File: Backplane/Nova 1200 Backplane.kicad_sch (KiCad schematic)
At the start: 46 parts, among them J1 Conn_02x40_Odd_Even, J10 Conn_01x10, J11 Conn_01x10, J12 Conn_01x10, J13 Conn_01x10, J14 Conn_01x10, J15 Conn_01x10, J16 Conn_01x10, J17 Conn_01x10, J18 Conn_01x10, J19 Conn_01x10, J1A1 Conn_01x40, J1A2 Conn_01x40, J1A3 Conn_01x40, J1A4 Conn_01x40, J1A5 Conn_01x40, J1B1 Conn_01x40, J1B2 Conn_01x40, J1B3 Conn_01x40, J1B4 Conn_01x40, J1B5 Conn_01x40, J2 DG Nova Card-Edge 81-100, J20 Conn_01x10, J21 Conn_01x10, J22 Conn_01x10, J23 Conn_01x10, J24 Conn_01x10, J2A1 Conn_01x40, J2A2 Conn_01x40, J2A3 Conn_01x40, J2A4 Conn_01x40, J2A5 Conn_01x40, J2B1 Conn_01x40, J2B2 Conn_01x40, J2B3 Conn_01x40, J2B4 Conn_01x40, J2B5 Conn_01x40, J3 Conn_02x40_Odd_Even, J4 DG Nova Card-Edge 81-100, J5 Conn_01x10, J6 Conn_01x10, J7 Conn_01x10, J8 Conn_01x10, J9 Conn_01x10

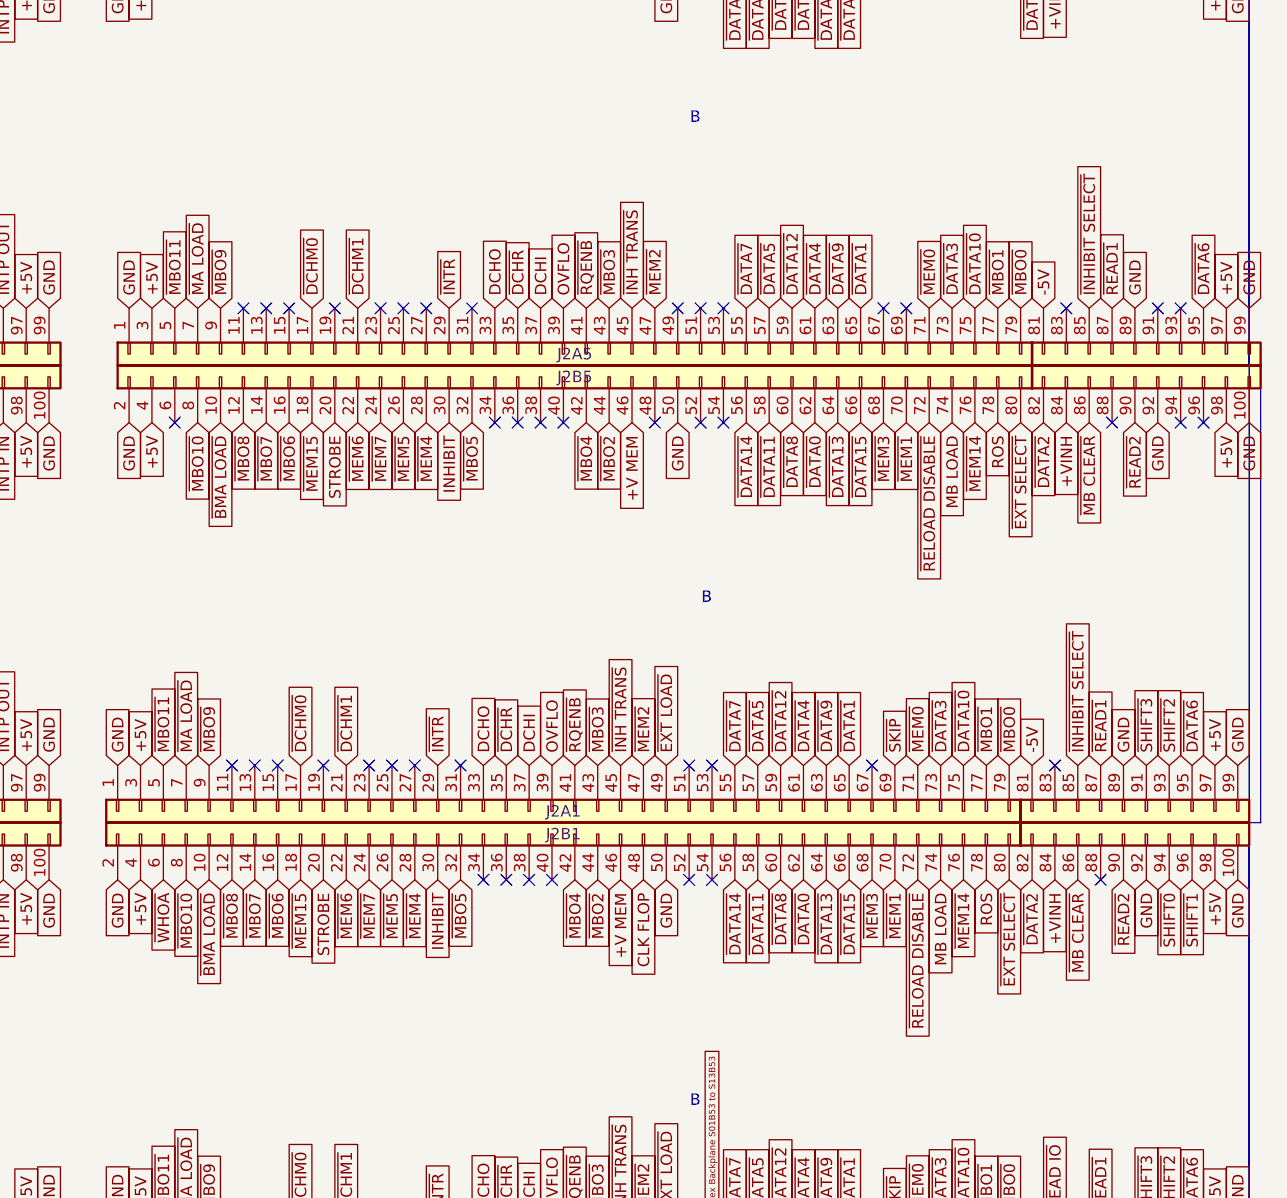
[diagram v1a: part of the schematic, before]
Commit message: more
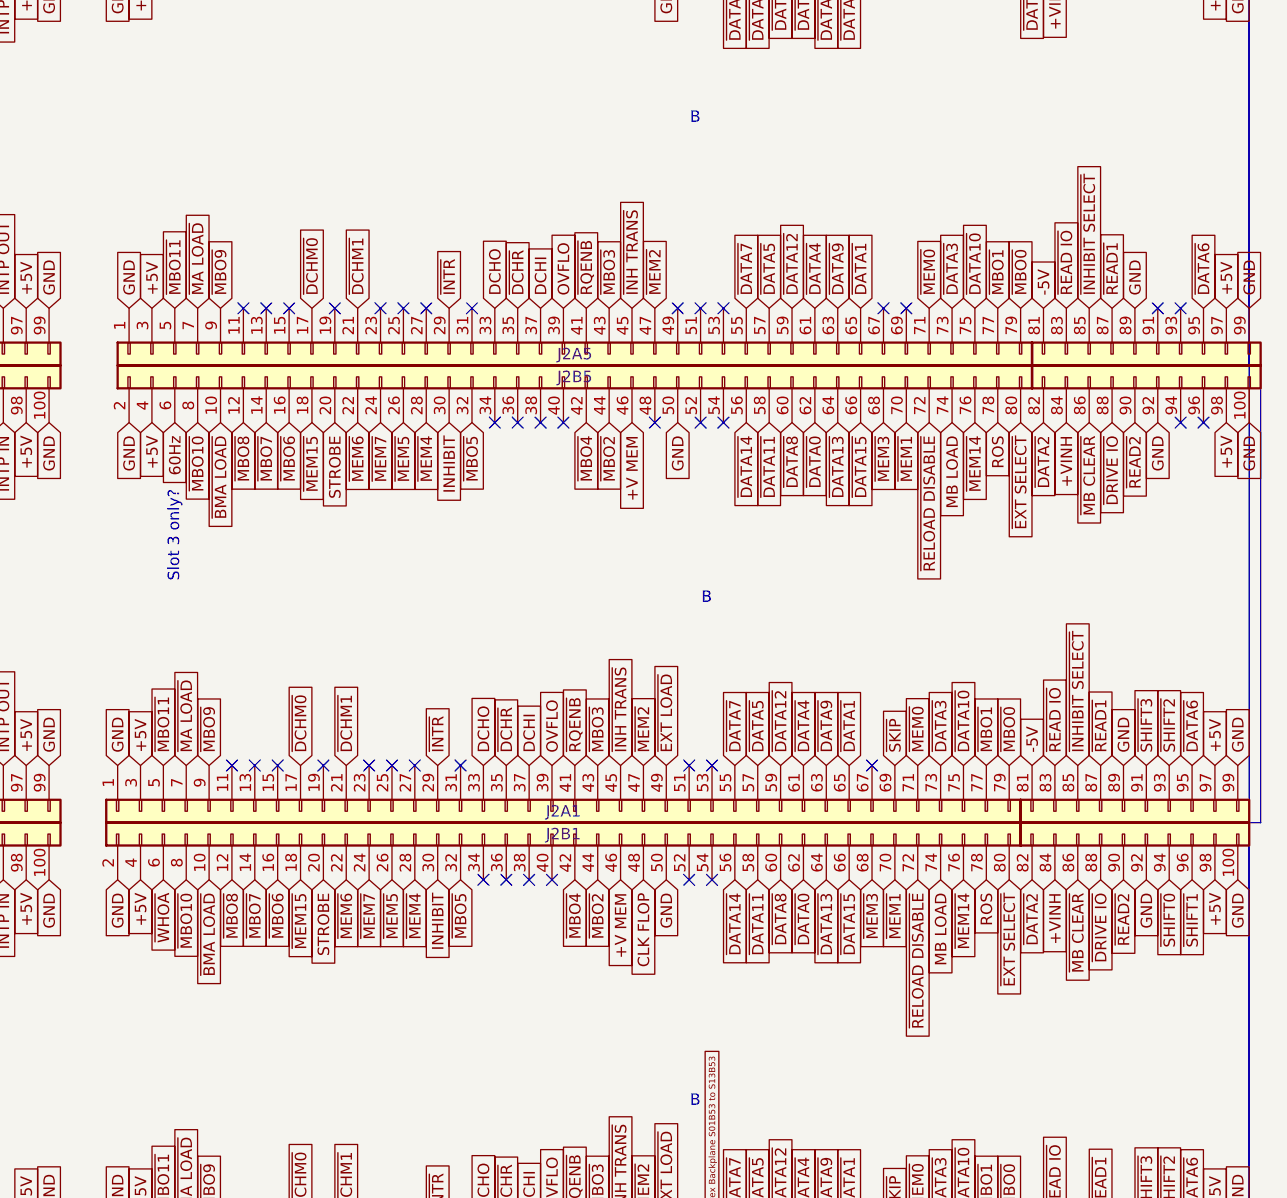
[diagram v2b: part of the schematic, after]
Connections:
- net ~{DRIVE IO}: now also J24.88 (Pin_4), J8.88 (Pin_4)
- net ~{READ IO}: now also J23.83, J7.83
- net 60Hz: now reaches J2B5.6
- no-connect marks 467 -> 462
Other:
- note added: "Slot 3 only?"
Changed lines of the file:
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@@
   (no_connect (at 254 238.76))
   (no_connect (at 248.92 149.86))
-  (no_connect (at 320.04 238.76))
   (no_connect (at 248.92 99.06))
   (no_connect (at 269.24 48.26))
@@
   (no_connect (at 279.4 86.36))
   (no_connect (at 251.46 48.26))
-  (no_connect (at 321.31 187.96))
   (no_connect (at 299.72 289.56))
   (no_connect (at 314.96 48.26))
@@
   (no_connect (at 200.66 302.26))
   (no_connect (at 177.8 149.86))
-  (no_connect (at 325.12 251.46))
   (no_connect (at 243.84 149.86))
   (no_connect (at 193.04 251.46))
@@
   (no_connect (at 185.42 137.16))
   (no_connect (at 312.42 35.56))
-  (no_connect (at 326.39 200.66))
   (no_connect (at 304.8 35.56))
   (no_connect (at 196.85 99.06))
@@
   (no_connect (at 300.99 187.96))
   (no_connect (at 228.6 149.86))
-  (no_connect (at 222.25 200.66))
   (no_connect (at 243.84 137.16))
   (no_connect (at 160.02 137.16))
@@
     (effects (font (size 1.27 1.27)) (justify left bottom))
   )
+  (text "Slot 3 only?" (at 222.885 208.28 90)
+    (effects (font (size 1.27 1.27)) (justify right bottom))
+  )
   (text "B" (at 280.035 61.595 0)
     (effects (font (size 1.27 1.27)) (justify right bottom))
@@
     )
   )
+  (global_label "~{READ IO}" (shape input) (at 321.31 187.96 90) (fields_autoplaced)
+    (effects (font (size 1.27 1.27)) (justify left))
+    (property "Intersheetrefs" "${INTERSHEET_REFS}" (at 321.31 177.5793 90)
+      (effects (font (size 1.27 1.27)) (justify left) hide)
+    )
+  )
   (global_label "+5V" (shape input) (at 204.47 99.06 270) (fields_autoplaced)
     (effects (font (size 1.27 1.27)) (justify right))
@@
     )
   )
+  (global_label "60Hz" (shape input) (at 222.25 200.66 270) (fields_autoplaced)
+    (effects (font (size 1.27 1.27)) (justify right))
+    (property "Intersheetrefs" "${INTERSHEET_REFS}" (at 222.25 208.3434 90)
+      (effects (font (size 1.27 1.27)) (justify right) hide)
+    )
+  )
   (global_label "DISK1" (shape input) (at 189.23 86.36 90) (fields_autoplaced)
     (effects (font (size 1.27 1.27)) (justify left))
@@
     )
   )
+  (global_label "~{READ IO}" (shape input) (at 320.04 238.76 90) (fields_autoplaced)
+    (effects (font (size 1.27 1.27)) (justify left))
+    (property "Intersheetrefs" "${INTERSHEET_REFS}" (at 320.04 228.3793 90)
+      (effects (font (size 1.27 1.27)) (justify left) hide)
+    )
+  )
   (global_label "RNIH4" (shape input) (at 99.06 187.96 90) (fields_autoplaced)
     (effects (font (size 1.27 1.27)) (justify left))
@@
     )
   )
+  (global_label "~{DRIVE IO}" (shape input) (at 326.39 200.66 270) (fields_autoplaced)
+    (effects (font (size 1.27 1.27)) (justify right))
+    (property "Intersheetrefs" "${INTERSHEET_REFS}" (at 326.39 211.6455 90)
+      (effects (font (size 1.27 1.27)) (justify right) hide)
+    )
+  )
   (global_label "GND" (shape input) (at 276.86 99.06 270) (fields_autoplaced)
     (effects (font (size 1.27 1.27)) (justify right))
@@
     )
   )
+  (global_label "~{DRIVE IO}" (shape input) (at 325.12 251.46 270) (fields_autoplaced)
+    (effects (font (size 1.27 1.27)) (justify right))
+    (property "Intersheetrefs" "${INTERSHEET_REFS}" (at 325.12 262.4455 90)
+      (effects (font (size 1.27 1.27)) (justify right) hide)
+    )
+  )
